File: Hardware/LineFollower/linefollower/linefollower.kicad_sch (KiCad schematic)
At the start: 6 parts, among them U1 OPB704, U2 74HC14

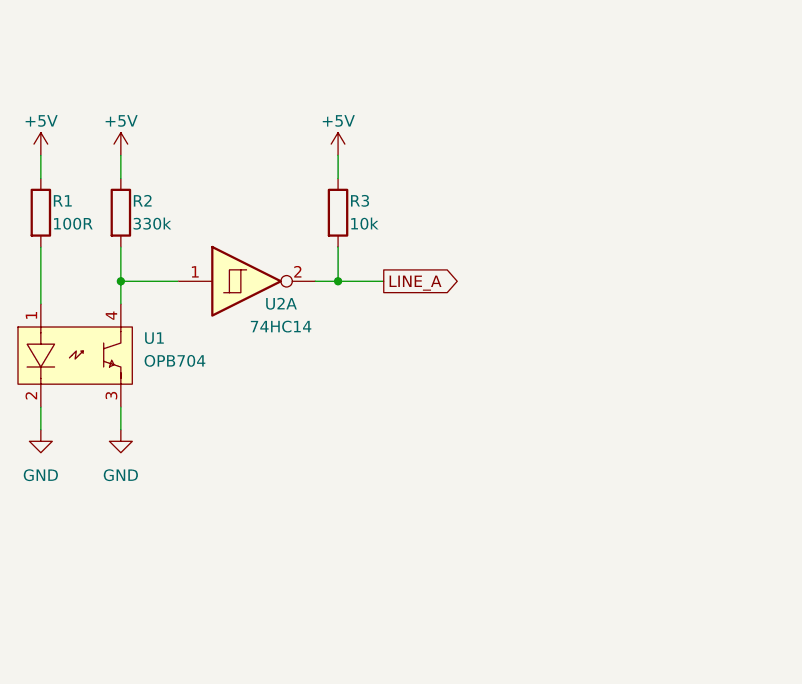
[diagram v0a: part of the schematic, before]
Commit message: linefollower
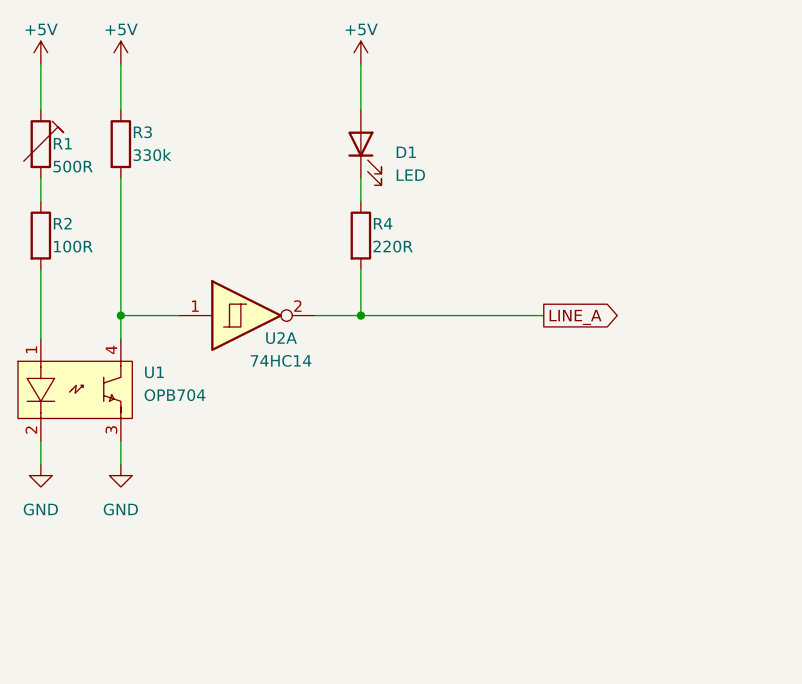
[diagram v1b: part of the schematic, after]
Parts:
- removed R3: 10k, symbol Device:R
- added D1: LED, symbol Device:LED
- added R1: 500R, symbol Device:R_Trim
- added R4: 220R, symbol Device:R
- renumbered R1 to R2, R2 to R3
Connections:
- net +5V: now also D1.2 (A), R1.1; no longer R2.1
- net LINE_A: now also R4.2
- new net: R1.2, R2.1
- new net: D1.1 (K), R4.1
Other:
- moved on the sheet: R2, R3, U1, U2A
